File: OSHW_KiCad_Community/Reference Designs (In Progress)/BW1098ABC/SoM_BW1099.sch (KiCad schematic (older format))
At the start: 25 parts, among them J1 20021121-00010T1LF, J2 20021121-00010T1LF, J3 DF40HC(3.0)-100DS-0.4V_BW1099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, J4 20021121-00010T1LF, Q1 BSS138LT1, Q2 BSS138LT1, Q3 BSS138LT1

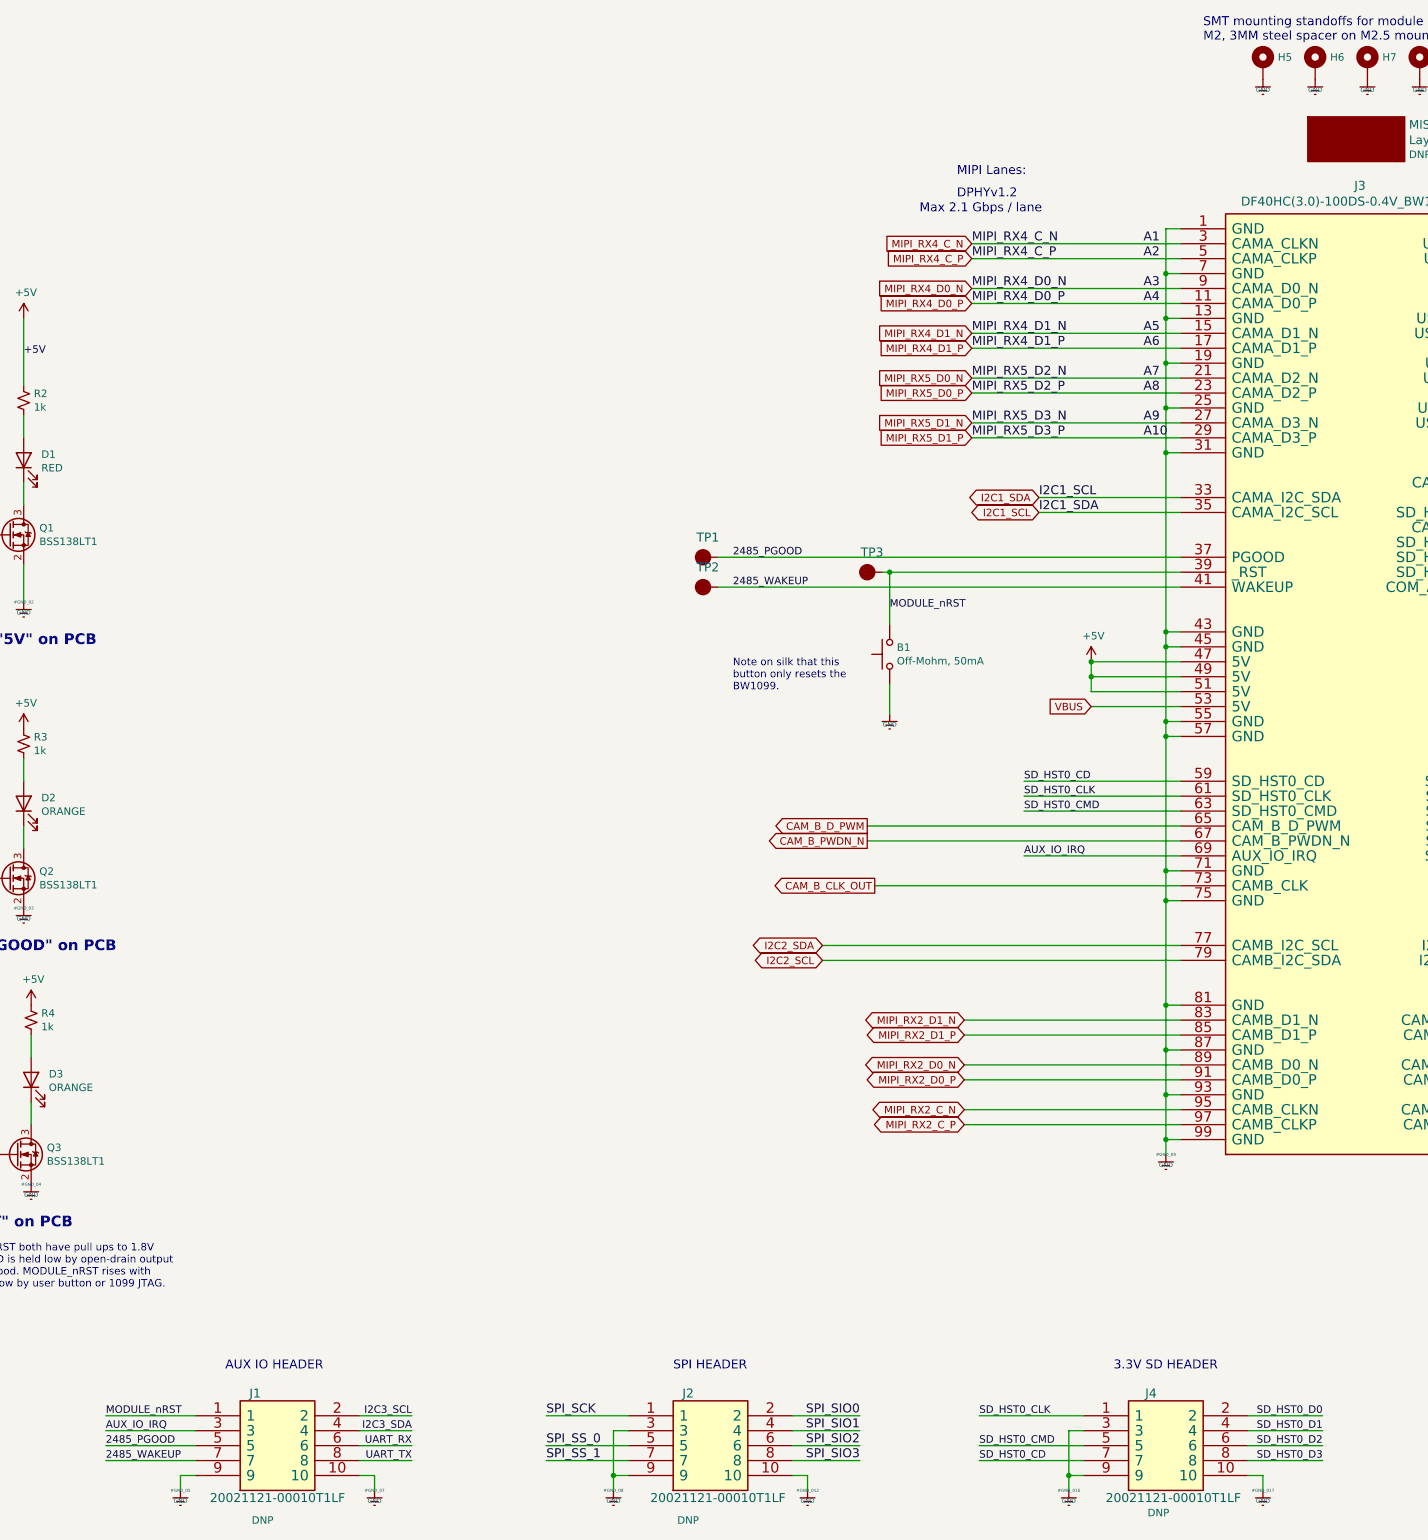
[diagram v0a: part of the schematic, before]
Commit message: abc board pcb work
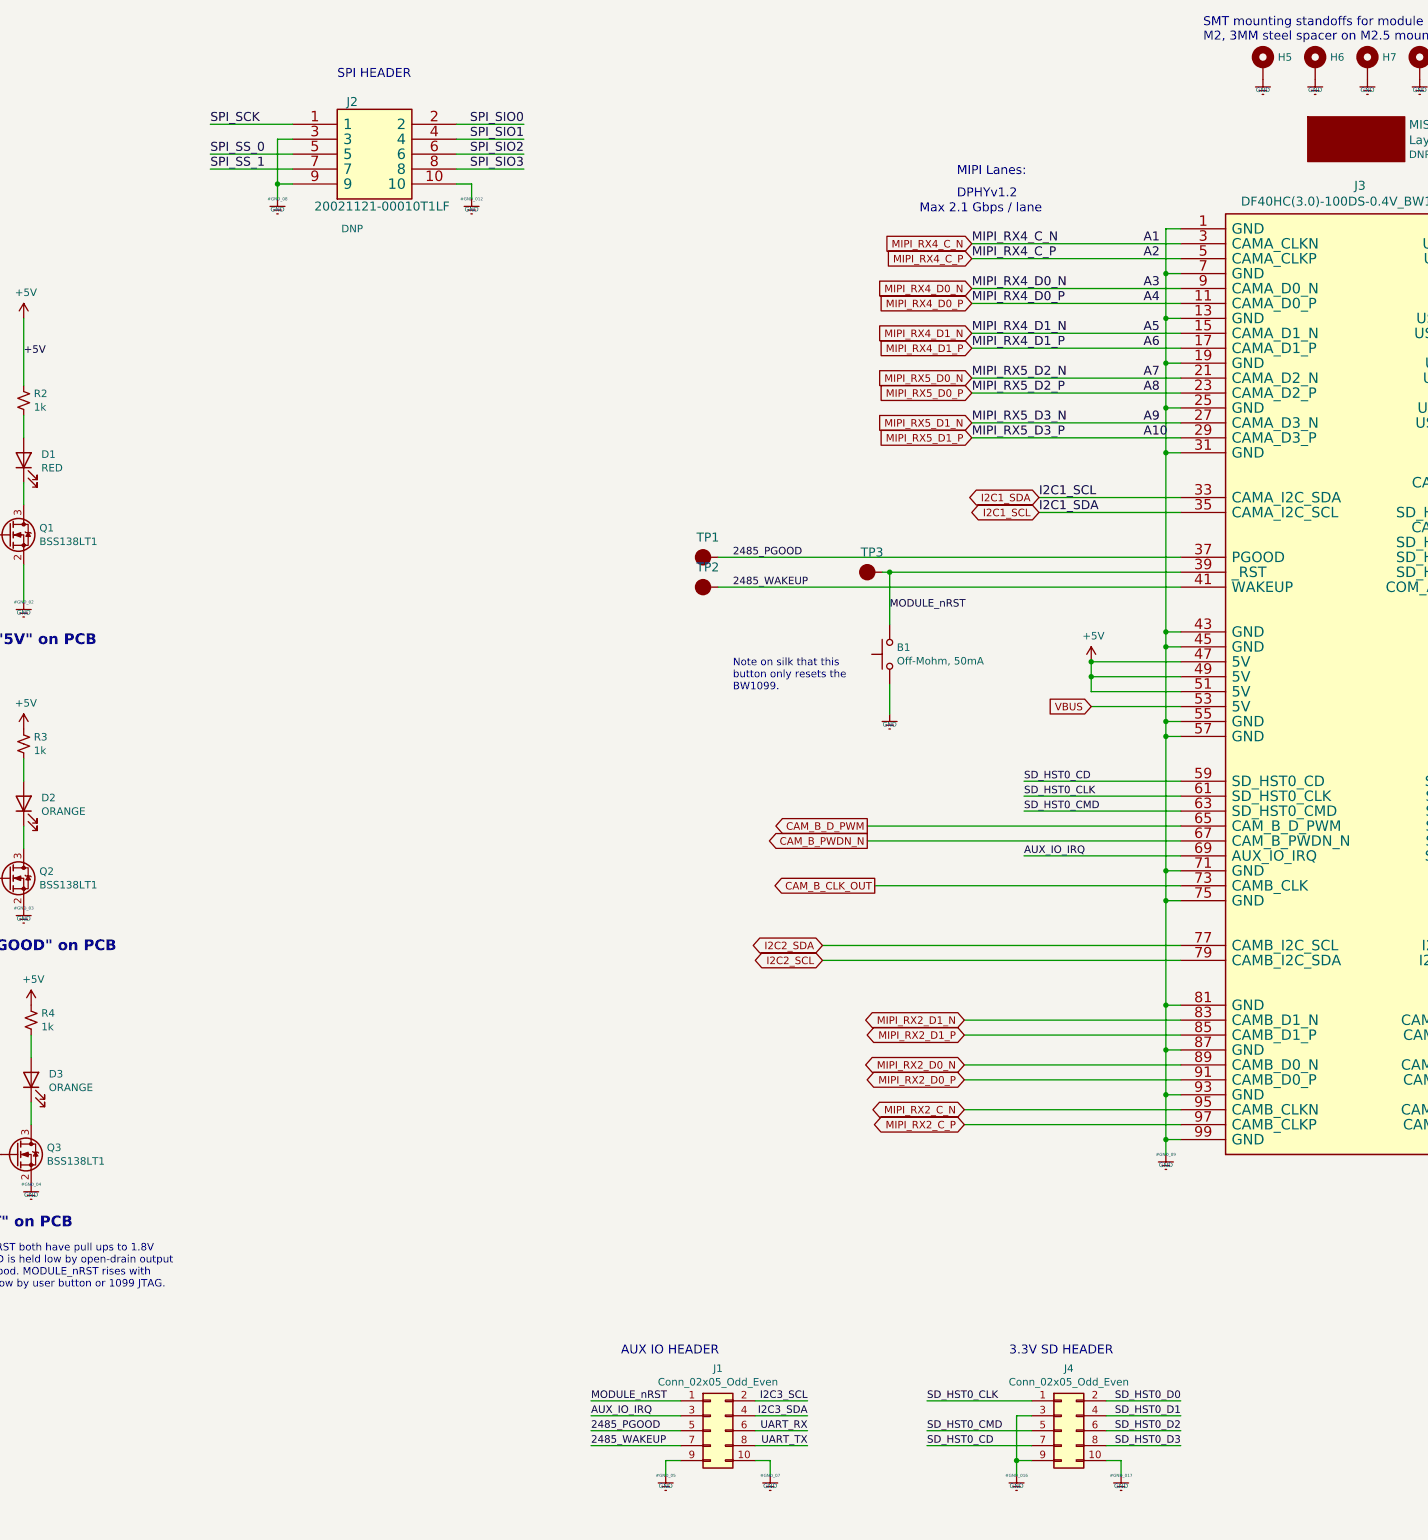
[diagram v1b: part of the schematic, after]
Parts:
- removed J1, J4: 20021121-00010T1LF, symbol BW1098ABC-rescue:20021121-00010T1LF-depthAI_sch
- added J1, J4: Conn_02x05_Odd_Even, Connector_PinSocket_2.54mm:PinSocket_2x05_P2.54mm_Vertical, symbol Connector_Generic:Conn_02x05_Odd_Even
- J2: footprint (none) -> Connector_PinHeader_2.54mm:PinHeader_1x02_P2.54mm_Vertical
- R1, R2, R3, R4: footprint Resistor_SMD:R_0402_1005Metric -> Resistor_SMD:R_0603_1608Metric
- TP1, TP2, TP3, TP4, TP5: footprint TestPoint:TestPoint_Loop_D1.80mm_Drill1.0mm_Beaded -> TestPoint:TestPoint_Pad_1.0x1.0mm
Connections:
- net 2485_PGOOD: now also J1.5 (Pin_5)
- net 2485_WAKEUP: now also J1.7 (Pin_7)
- net AUX_IO_IRQ: now also J1.3 (Pin_3)
- net Earth: now also J1.10 (Pin_10), J1.9 (Pin_9), J4.10 (Pin_10), J4.3 (Pin_3), J4.9 (Pin_9)
- net I2C3_SCL: now also J1.2 (Pin_2)
- net I2C3_SDA: now also J1.4 (Pin_4)
- net MODULE_nRST: now also J1.1 (Pin_1)
- net SD_HST0_CD: now also J4.7 (Pin_7)
- net SD_HST0_CLK: now also J4.1 (Pin_1)
- net SD_HST0_CMD: now also J4.5 (Pin_5)
- net SD_HST0_D0: now also J4.2 (Pin_2)
- net SD_HST0_D1: now also J4.4 (Pin_4)
- net SD_HST0_D2: now also J4.6 (Pin_6)
- net SD_HST0_D3: now also J4.8 (Pin_8)
- net UART_RX: now also J1.6 (Pin_6)
- net UART_TX: now also J1.8 (Pin_8)
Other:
- moved on the sheet: J2

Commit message: layout
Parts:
- removed J2: 20021121-00010T1LF, Connector_PinHeader_2.54mm:PinHeader_1x02_P2.54mm_Vertical, symbol BW1098ABC-rescue:20021121-00010T1LF-depthAI_sch
- removed TP2, TP3: TEST_POINT, TestPoint:TestPoint_Pad_1.0x1.0mm, symbol BW1098ABC-rescue:TEST_POINT-depthAI_sch
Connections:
- net 2485_PGOOD: no longer J1.5 (Pin_5)
- net I2C1_SCL: no longer J3.33 (CAMA_I2C_SDA)
- net I2C3_SCL: no longer J1.2 (Pin_2)
- net I2C3_SDA: no longer J1.4 (Pin_4)
- net 2485_WAKEUP: no longer names the net of J3.41 (WAKEUP)
- net 2485_WAKEUP: no longer J1.7 (Pin_7)
- net MODULE_nRST renamed _RST
- net SPI_SS_0 renamed SPI_CS_0
- net SPI_SS_1 renamed SPI_CS_1
- new net I2C1_SDA: J3.33 (CAMA_I2C_SDA)
- no-connect marks 0 -> 1
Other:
- note added: "ALL PU/PD on SoM,\nSee Datasheet"
- note added: "DO NOT USE SPI0_CS_0 for \nanother peripheral IF \nyou are using the BW1099EMB\nit selects the nor flash"
- note added: "SPI0_SIO2&3 have 10k pullup on SoM"
- note removed: "SPI HEADER"
- moved on the sheet: B1, D1, D2, D3, H5, H6, H7, H8, J1, J3, J4, MISC1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

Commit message: ABC Updates
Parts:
- added D4, D5: RED, Diode_SMD:D_0603_1608Metric, symbol Device:LED
- added Q4, Q5: BSS138LT1, Package_TO_SOT_SMD:SOT-23, symbol Device:Q_NMOS_GSD
- added R29, R35: 100, Resistor_SMD:R_0603_1608Metric, symbol Device:R_Small_US
- added R30, R36: 1k, Resistor_SMD:R_0603_1608Metric, symbol Device:R_Small_US
- added R33, R34, R37: 10k, Resistor_SMD:R_0603_1608Metric, symbol Device:R_Small_US
- B1: footprint Luxonis_KiCad_Master:DTSM32NVTR -> depthABC:SW_PTS636_SM43J_SMTR_LFS; symbol Switch:SW_MEC_5G -> Switch:SW_SPST
- J1, J4: footprint Connector_PinSocket_2.54mm:PinSocket_2x05_P2.54mm_Vertical -> Connector_PinSocket_2.54mm:PinSocket_2x05_P2.54mm_Vertical_SMD
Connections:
- net +5V: now also R30.1, R36.1
- net Earth: now also Q4.2 (S), Q5.2 (S), R33.2, R34.2, R37.2; no longer B1.2 (A)
- net I2C3_SCL: now also J1.7 (Pin_7)
- net I2C3_SDA: now also J1.5 (Pin_5)
- net _RST: now also B1.2 (B); no longer B1.3 (B), B1.4 (B)
- net at Q1.1 (G), R1.2: now also R34.1
- net 1V8: now reaches J1.2 (Pin_2)
- net 1V8: now also J1.4 (Pin_4), R35.1
- net MIPI_RX5_D0_N renamed MIPI_RX5_D2_N
- net MIPI_RX5_D0_P renamed MIPI_RX5_D2_P
- net MIPI_RX5_D1_N renamed MIPI_RX5_D3_N
- net MIPI_RX5_D1_P renamed MIPI_RX5_D3_P
- new net: Q4.1 (G), R29.2, R33.1
- new net: D5.1 (K), Q5.3 (D)
- new net: D5.2 (A), R36.2
- new net: Q5.1 (G), R35.2, R37.1
- new net: D4.1 (K), Q4.3 (D)
- new net: D4.2 (A), R30.2
- new net +3V3: R29.1
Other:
- moved on the sheet: D1, D2, D3, J1, J3, MISC1, Q1, Q2, Q3, R1, R2, R3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
